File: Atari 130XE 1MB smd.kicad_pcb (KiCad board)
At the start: 2 copper layers, 324 x 204 mm, 369 parts, among them J1 SIO, J10 Mem_on_off, J2 Video, J201 Diagnostic, J202 Diag, J210 Diag, J24 Cartridge, J4 Expansion, J5 Joystick_Port, J50 Test_signal, J500 Basic_sel, J501 TPP_sel, J51 To_GND, J6 Joystick_Port, J7 Power, J8 Keyboard, Q1 2N3904, Q10 PN2222A, Q101 BC849, Q11 PN2222A, Q2 2N3904, Q3 2N3904, Q4 2N3906, Q6 2N3904, SW1 Switch_power_on, U10 DRAM_4464, U100 74LS157, U101 74LS74, U102 74HC02, U103 74HC02, U104 74LS157, U105 74HC74, U17 GTIA, U18 74LS08, U19 LM555, U2 74LS138, U20 4050, U21 74LS74, U22 POKEY, U23 PIA, U24 CD4051B, U25 CD4051B, U3 MMU, U4 27C010, U40 GAL20V8_DIP, U41 74LS157, U42 74LS175, U43 DRAM_1MB_4bit, U44 DRAM_1MB_4bit, U45 74HC04, U5 27C010, U6 Freddie, U7 Antic, U8 Sally, U9 DRAM_4464, Y1 Crystal, Y2 4,43 MHz

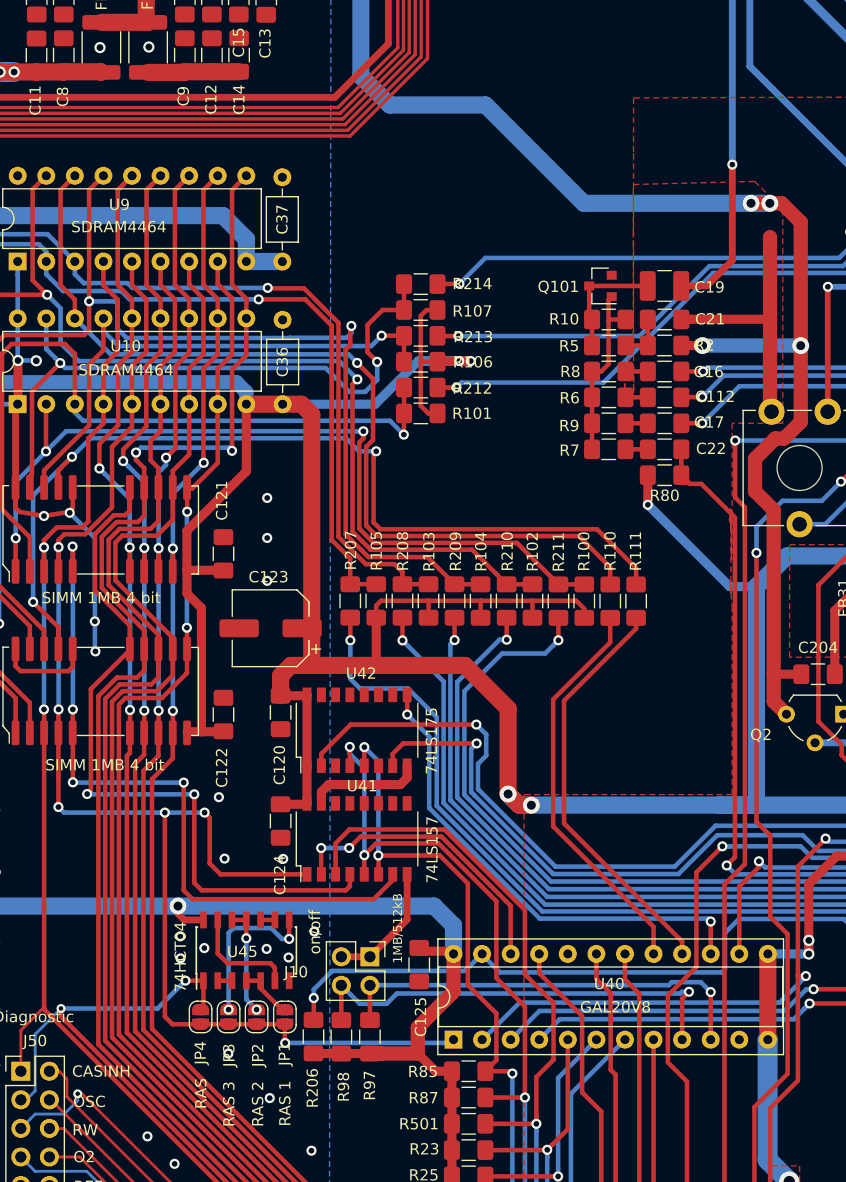
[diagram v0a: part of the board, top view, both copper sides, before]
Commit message: Gerber
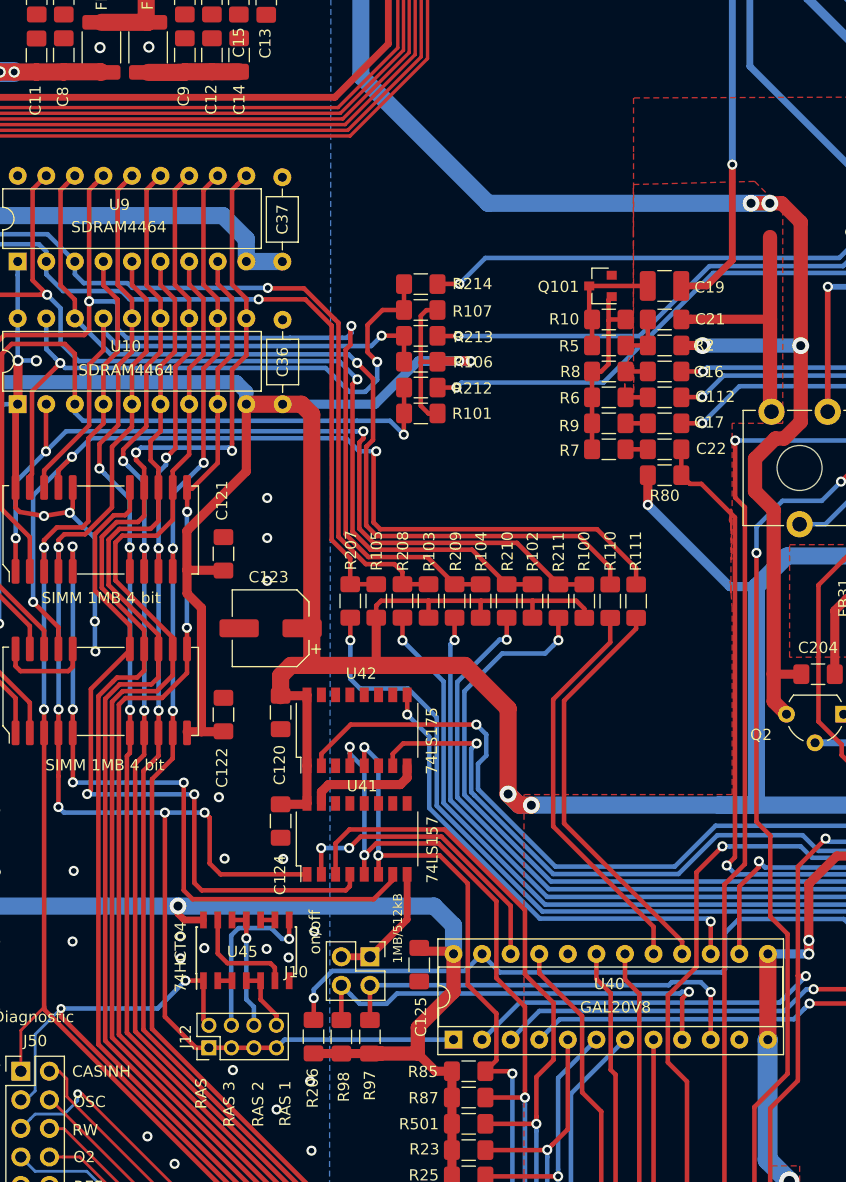
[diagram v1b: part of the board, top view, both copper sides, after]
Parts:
- removed JP1, JP2, JP3, JP4: SolderJumper_2_Open, Jumper:SolderJumper-2_P1.3mm_Open_RoundedPad1.0x1.5mm
- added J12: Conn_02x04_Odd_Even, Connector_PinHeader_2.00mm:PinHeader_2x04_P2.00mm_Vertical, F.Cu at (81.4, 181.4)
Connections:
- U20 pad 16: +5VA -> (no net)
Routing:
- net RAS: track 66.5 -> 68.0 mm
- net Net-(J12-Pad6): track 9.62 -> 10.9 mm, vias 2 -> 1
- net Net-(J12-Pad4): track 14.5 -> 15.5 mm, vias 2 -> 1
- net Net-(J12-Pad8): track 4.89 -> 5.81 mm
- net RAS_out: track 128.2 -> 127.6 mm, vias 6 -> 5
- net GND: vias 164 -> 167
